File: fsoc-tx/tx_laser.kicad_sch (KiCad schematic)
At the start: 0 parts

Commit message: TX ROOT: laser + host IO
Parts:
- added C21: 100 nF, symbol Device:C
- added C22: 1 µF, symbol Device:C
- added J4: B3B-PH-K-S, Connector_JST:JST_PH_B3B-PH-K_1x03_P2.00mm_Vertical, symbol fsoc_symbols:B3B-PH-K-S
- added MOD1: ARD-LASER-MDI650-1-5, symbol fsoc_symbols:ARD-LASER-MDI650-1-5
- added R10, R9: 100 kΩ, symbol Device:R
- added R11, R8: 10 kΩ, symbol Device:R
- added SW3: SW_DPST, symbol Switch:SW_DPST
- added U4: 74AHCT1G125, symbol 74xGxx:74AHCT1G125
- added U5: TPS22919DCK, Package_TO_SOT_SMD:SOT-363_SC-70-6, symbol Power_Management:TPS22919DCK
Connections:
- new net: R10.1, SW3.2, U5.3 (ON)
- new net: R8.2, SW3.3, U4.1
- new net GND: C21.1, C22.2, J4.2 (Pin_2), MOD1.2 (GND), R10.2, R11.2, R9.2, SW3.4, U4.3 (GND), U5.2 (GND)
- new net LASER_DATA_3V3: R9.1, U4.2
- new net LASER_DATA_5V: J4.3 (Pin_3), MOD1.3 (MOD), R11.1, U4.4
- new net LASER_MODULE_5V: J4.1 (Pin_1), MOD1.1 (VDD), U5.5 (QOD), U5.6 (OUT)
- new net LASER_PWR_EN: SW3.1
- new net SYS_5V: C21.2, C22.1, R8.1, U4.5 (VCC), U5.1 (IN)

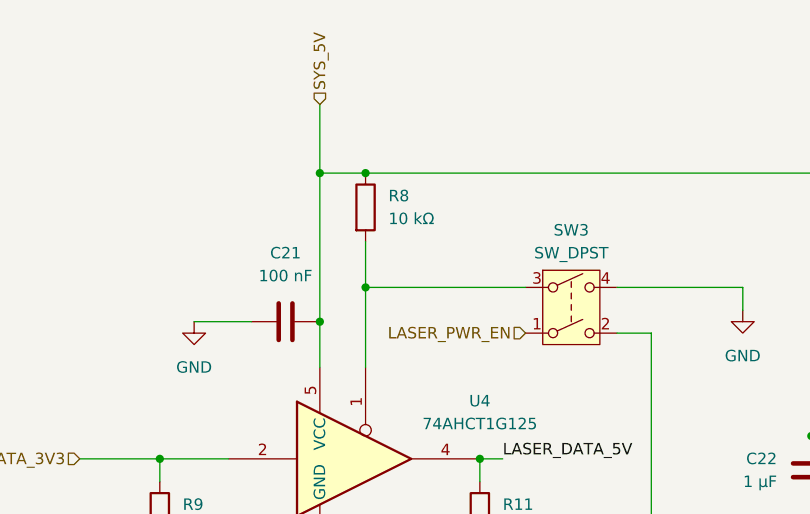
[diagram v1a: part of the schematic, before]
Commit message: TX: fixing unassigned footprints
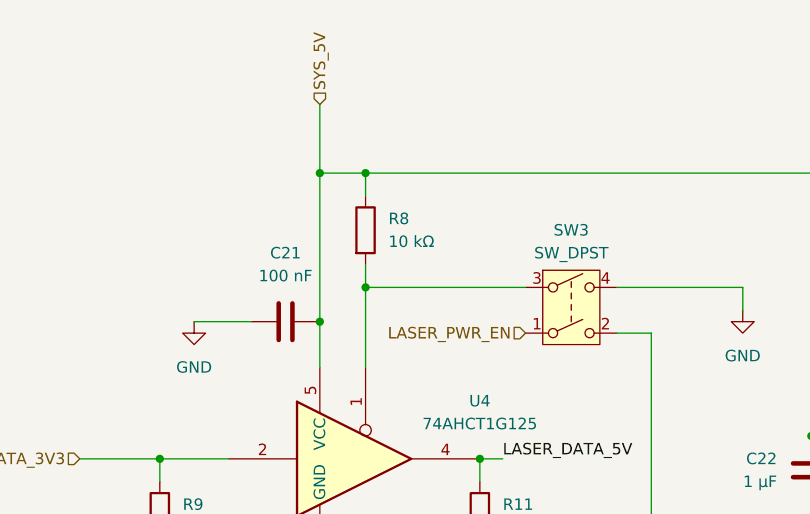
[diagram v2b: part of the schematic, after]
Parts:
- C21: footprint (none) -> Capacitor_SMD:C_0603_1608Metric
- C22: footprint (none) -> Capacitor_SMD:C_0805_2012Metric
- R10, R11, R8, R9: footprint (none) -> Resistor_SMD:R_0603_1608Metric
- SW3: footprint (none) -> fsoc_footprints:ES22MCBE
- U4: footprint (none) -> Package_TO_SOT_SMD:SOT-23-5
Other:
- moved on the sheet: R8
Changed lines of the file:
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@@
 	(paper "A4")
+	(junction
+		(at 87.63 67.31)
+		(diameter 0)
+		(color 0 0 0 0)
+	)
 	(junction
 		(at 92.71 80.01)
@@
 	)
 	(junction
-		(at 87.63 67.31)
-		(diameter 0)
-		(color 0 0 0 0)
-	)
-	(junction
 		(at 87.63 83.82)
 		(diameter 0)
@@
 	)
 	(junction
-		(at 92.71 67.31)
-		(diameter 0)
-		(color 0 0 0 0)
-	)
-	(junction
 		(at 105.41 99.06)
 		(diameter 0)
@@
 		(color 0 0 0 0)
 	)
-	(wire
-		(pts
-			(xy 92.71 74.93) (xy 92.71 80.01)
+	(junction
+		(at 92.71 67.31)
+		(diameter 0)
+		(color 0 0 0 0)
+	)
+	(wire
+		(pts
+			(xy 92.71 77.47) (xy 92.71 80.01)
 		)
 		(stroke
@@
 		(pts
 			(xy 146.05 111.76) (xy 146.05 101.6)
+		)
+		(stroke
+			(width 0)
+			(type default)
+		)
+	)
+	(wire
+		(pts
+			(xy 92.71 69.85) (xy 92.71 67.31)
 		)
 		(stroke
@@
 			)
 		)
-		(property "Footprint" ""
+		(property "Footprint" "Capacitor_SMD:C_0603_1608Metric"
 			(at 87.63 82.8548 0)
 			(hide yes)
@@
 	(symbol
 		(lib_id "Device:R")
-		(at 92.71 71.12 0)
+		(at 92.71 73.66 0)
 		(unit 1)
 		(body_style 1)
@@
 		(fields_autoplaced yes)
 		(property "Reference" "R8"
-			(at 95.25 69.8499 0)
+			(at 95.25 72.3899 0)
 			(show_name no)
 			(do_not_autoplace no)
@@
 		)
 		(property "Value" "10 kΩ"
-			(at 95.25 72.3899 0)
+			(at 95.25 74.9299 0)
 			(show_name no)
 			(do_not_autoplace no)
@@
 			)
 		)
-		(property "Footprint" ""
-			(at 90.932 71.12 90)
+		(property "Footprint" "Resistor_SMD:R_0603_1608Metric"
+			(at 90.932 73.66 90)
 			(hide yes)
 			(show_name no)
@@
 		)
 		(property "Datasheet" ""
-			(at 92.71 71.12 0)
+			(at 92.71 73.66 0)
 			(hide yes)
 			(show_name no)
@@
 		)
 		(property "Description" "Resistor"
-			(at 92.71 71.12 0)
+			(at 92.71 73.66 0)
 			(hide yes)
 			(show_name no)
@@
 			)
 		)
-		(property "Footprint" ""
+		(property "Footprint" "Resistor_SMD:R_0603_1608Metric"
 			(at 68.072 105.41 90)
 			(hide yes)
@@
 			)
 		)
-		(property "Footprint" ""
+		(property "Footprint" "Resistor_SMD:R_0603_1608Metric"
 			(at 144.272 118.11 90)
 			(hide yes)
@@
 			)
 		)
-		(property "Footprint" ""
+		(property "Footprint" "Resistor_SMD:R_0603_1608Metric"
 			(at 103.632 105.41 90)
 			(hide yes)
@@
 			)
 		)
-		(property "Footprint" ""
+		(property "Footprint" "fsoc_footprints:ES22MCBE"
 			(at 115.57 82.55 0)
 			(hide yes)
@@
 			)
 		)
-		(property "Footprint" ""
+		(property "Footprint" "Package_TO_SOT_SMD:SOT-23-5"
 			(at 92.71 99.06 0)
 			(hide yes)
@@
 			)
 		)
-		(property "Footprint" ""
+		(property "Footprint" "Capacitor_SMD:C_0805_2012Metric"
 			(at 141.2748 104.14 0)
 			(hide yes)

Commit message: manufacturing files
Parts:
- J4: footprint Connector_JST:JST_PH_B3B-PH-K_1x03_P2.00mm_Vertical -> Connector_PinHeader_2.54mm:PinHeader_1x03_P2.54mm_Vertical
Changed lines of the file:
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@@
 			)
 		)
-		(property "Footprint" "Connector_JST:JST_PH_B3B-PH-K_1x03_P2.00mm_Vertical"
+		(property "Footprint" "Connector_PinHeader_2.54mm:PinHeader_1x03_P2.54mm_Vertical"
 			(at 224.79 92.71 0)
 			(hide yes)
